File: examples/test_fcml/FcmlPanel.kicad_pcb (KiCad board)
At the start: 2 copper layers, 109 x 72 mm, 243 parts, among them J1 COM-15111 (Sparkfun), J2 COM-15111 (Sparkfun), J3 B2B-PH-K (JST), J4 B2B-PH-K (JST), J5 PinHeader1.27 Shrouded 2x5 (G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, J6 PinHeader1.27 Shrouded 2x5 (G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, Q1 HSM4410 (HUASHUO) - 30V 12A 2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, Q2 HSM4410 (HUASHUO) - 30V 12A 2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, Q3 HSM4410 (HUASHUO) - 30V 12A 2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, Q4 HSM4410 (HUASHUO) - 30V 12A 2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, Q5 HSM4410 (HUASHUO) - 30V 12A 2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, Q6 HSM4410 (HUASHUO) - 30V 12A 2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, SW1 5.1mm switch, SW2 5.1mm switch, U1 LD1117S33TR (STMicroelectroni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, U10 ICE40UP5K-SG48 (Lattice Semic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, U11 LD1117S12TR (STMicroelectroni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, U12 W25Q128JVSIQ (Winbond Electro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, U13 PGB102ST23 (Littelfuse), U14 RP2040 (Raspberry Pi), U15 W25Q128JVSIQ (Winbond Electro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, U16 PGB102ST23 (Littelfuse), U17 Duck, U18 Lemur, U19 IdDots4, U2 AP3012K (Diodes Incorporated), U3 IR2301 (Infineon Technologies), U4 AP2204K-3.3 (Diodes Incorpora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, U5 CBMuD1200L (Corebai), U6 IR2301 (Infineon Technologies), U7 AP2204K-3.3 (Diodes Incorpora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, U8 CBMuD1200L (Corebai), U9 IR2301 (Infineon Technologies)

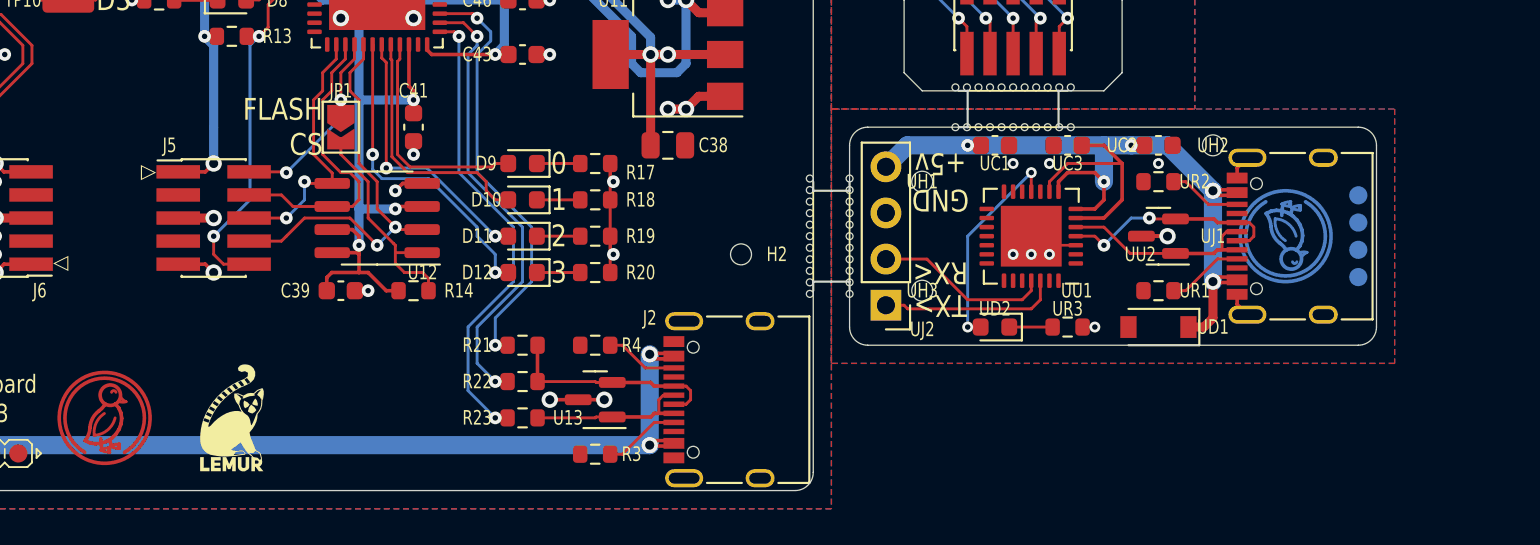
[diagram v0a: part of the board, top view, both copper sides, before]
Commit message: update
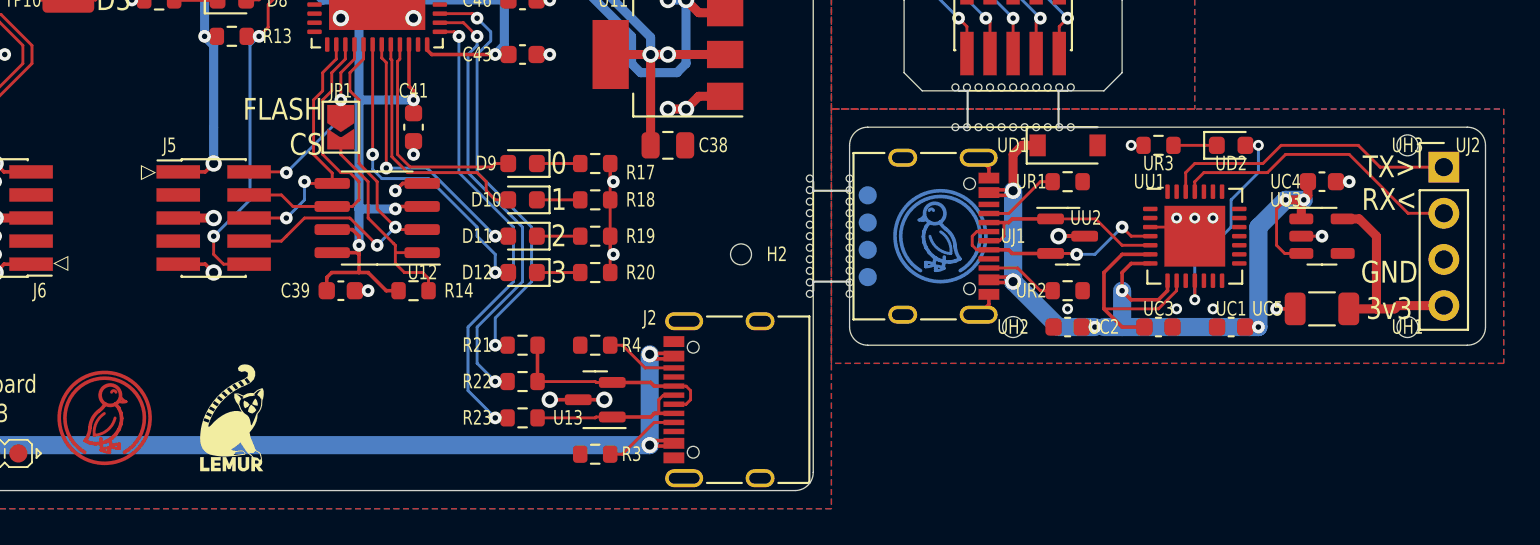
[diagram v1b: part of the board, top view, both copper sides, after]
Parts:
- added UC4: , Capacitor_SMD:C_0603_1608Metric, F.Cu at (132.0, 156.0)
- added UC5: , Capacitor_SMD:C_1206_3216Metric, F.Cu at (132.0, 163.0)
- added UU6: IdDots4, edg:Indicator_IdDots_4, B.Cu at (107.0, 159.0)
- UU3: value Duck -> AP2204K-3.3 (Diodes Incorporated); footprint edg:Symbol_Duckling -> Package_TO_SOT_SMD:SOT-23-5; moved to F.Cu
- UU4: value Lemur -> Duck; footprint edg:Symbol_LemurSmall -> edg:Symbol_Duckling
- UU5: value IdDots4 -> Lemur; footprint edg:Indicator_IdDots_4 -> edg:Symbol_LemurSmall
- moved UJ2 31.6 mm to (138.7, 155.2), turned to 0 degrees
- moved UH1 27.9 mm to (136.7, 164.0), turned to 0 degrees
- moved UH3 27.9 mm to (136.7, 154.0), turned to 0 degrees
- moved UJ1 21.0 mm to (110.0, 159.0), turned to -90 degrees
- moved UU5 18.0 mm to (116.0, 159.0), turned to 180 degrees
- moved UC1 16.4 mm to (127.0, 164.0), turned to 180 degrees
- moved UD2 16.4 mm to (127.0, 154.0), turned to 0 degrees
- moved UH2 14.9 mm to (115.0, 164.0), turned to 0 degrees
- moved UU4 14.0 mm to (111.0, 159.0), turned to 180 degrees
- moved UC2 11.2 mm to (118.0, 164.0), turned to 180 degrees
- moved UC3 11.2 mm to (123.0, 164.0), turned to 0 degrees
- moved UD1 11.2 mm to (118.0, 154.0), turned to 0 degrees
- moved UR3 11.2 mm to (123.0, 154.0), turned to 180 degrees
- moved UU1 9.00 mm to (125.0, 159.0), turned to 0 degrees
- moved UR1 7.81 mm to (118.0, 156.0), turned to 180 degrees
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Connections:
- UJ2 pad 4: vusb -> v3v3
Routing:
- net (no net): track 453.9 -> 466.9 mm
- net v3v3: track 367.2 -> 378.7 mm
- net vusb: track 237.1 -> 247.1 mm, vias 17 -> 19
- net gnd: track 149.6 -> 152.5 mm, vias 110 -> 113
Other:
- board size 109 x 72 mm -> 115 x 72 mm
- board text added: "3v3"
- board text removed: "+5v"
